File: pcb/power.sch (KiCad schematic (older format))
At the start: 46 parts, among them P11 CONN_01X01, P12 CONN_01X01, P8 CONN_01X06, P9 CONN_01X02, T1 NET-TIE, T2 NET-TIE, U1 TPS2420, U2 LT3487, U3 TPS63002, U7 TPS56x200, U8 LMZ10500

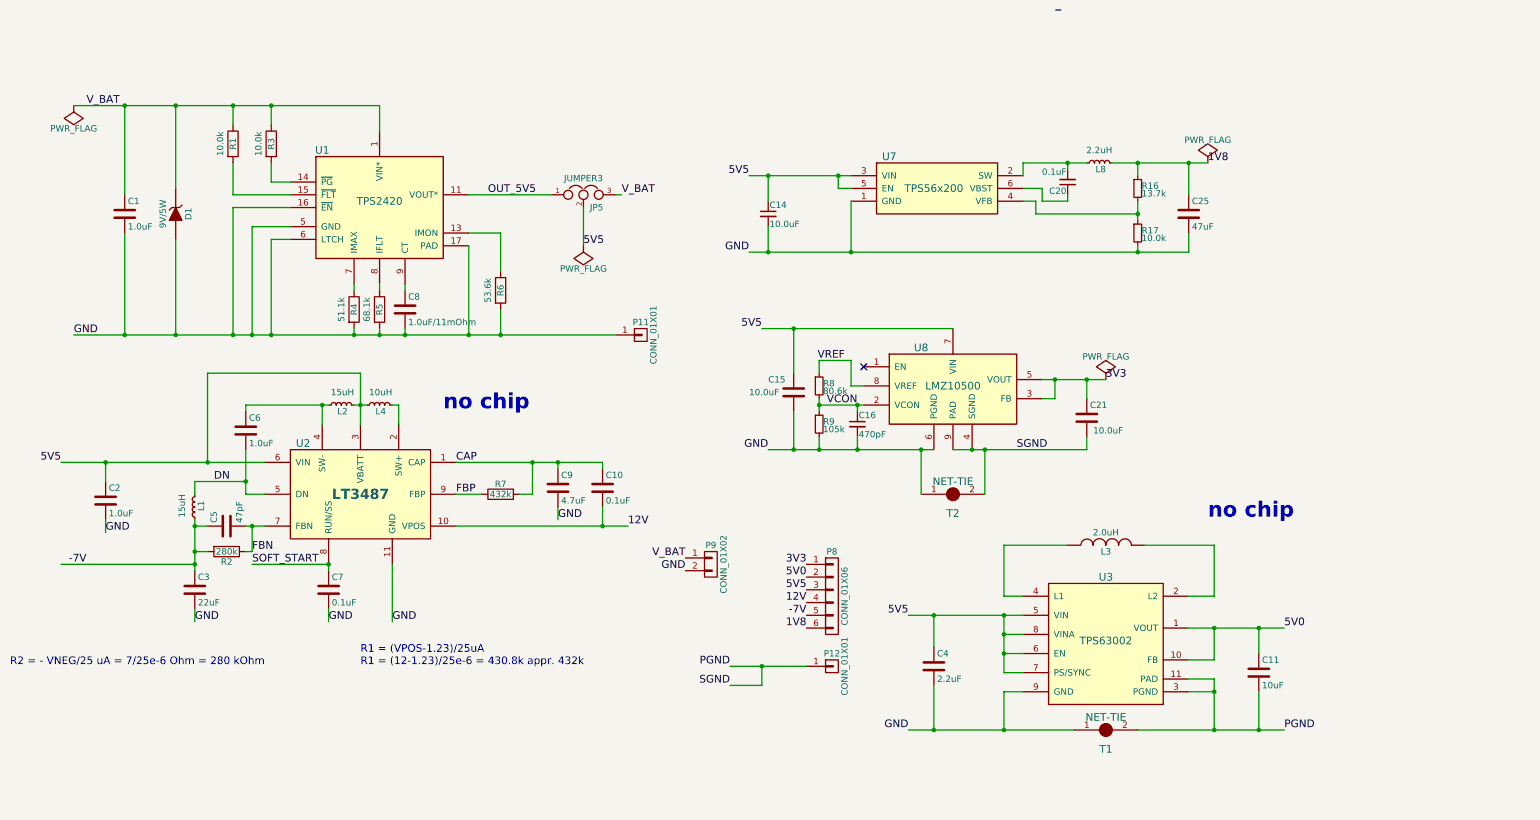
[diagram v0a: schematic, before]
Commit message: work
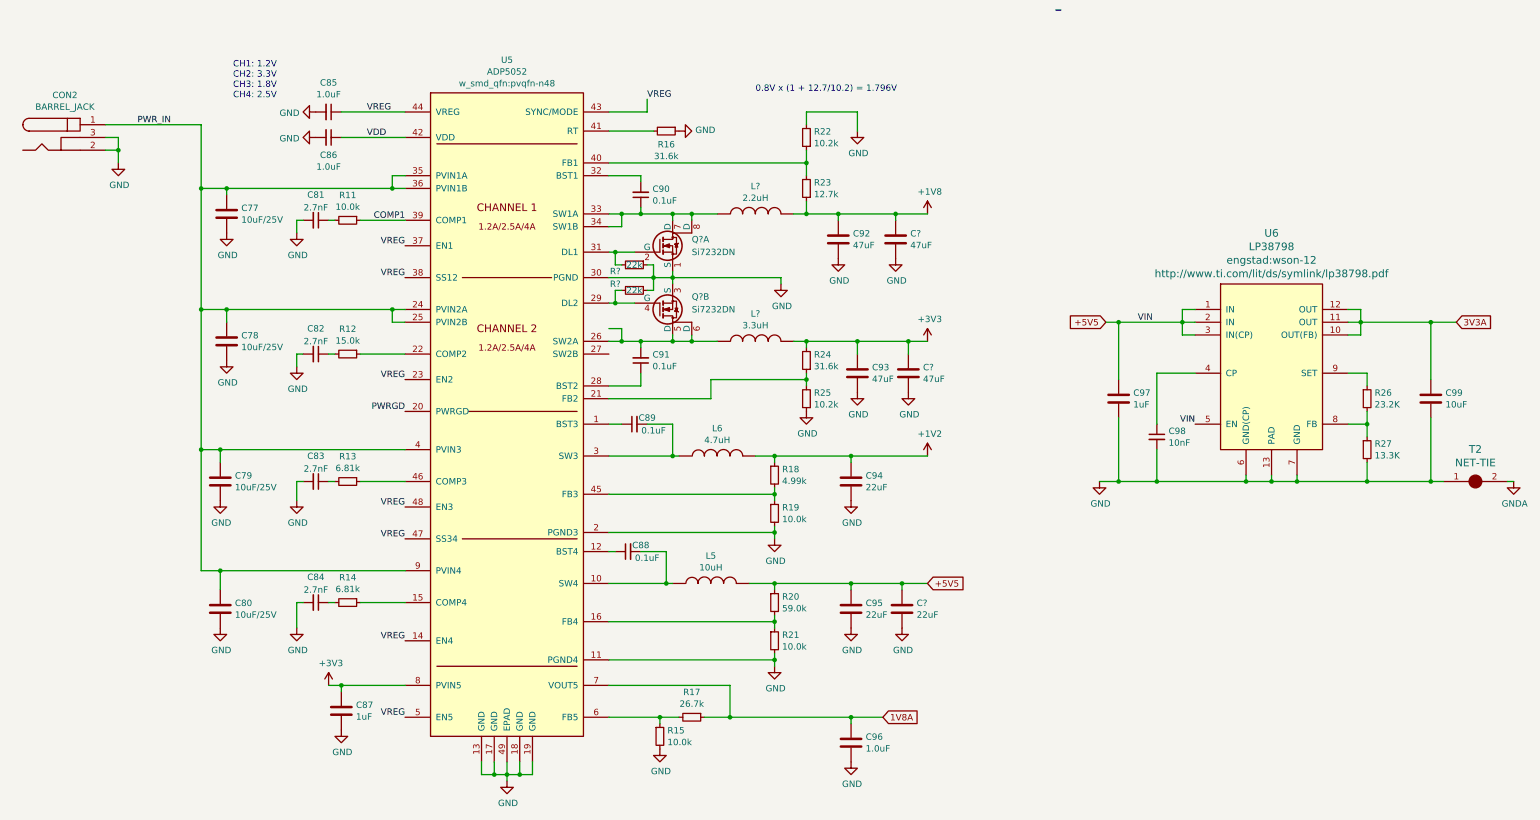
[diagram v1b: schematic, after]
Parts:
- removed C1, C2, C6: 1.0uF, Capacitors_SMD:C_0805_HandSoldering, symbol C
- removed C10, C7: 0.1uF, Capacitors_SMD:C_0805_HandSoldering, symbol C
- removed C11: 10uF, Capacitors_SMD:C_0805_HandSoldering, symbol C
- removed C14: 10.0uF, Capacitors_SMD:C_0805_HandSoldering, symbol C_Small
- removed C15, C21: 10.0uF, Capacitors_SMD:C_0805_HandSoldering, symbol C
- removed C16: 470pF, Capacitors_SMD:C_0402, symbol C_Small
- removed C20: 0.1uF, Capacitors_SMD:C_0603_HandSoldering, symbol C_Small
- removed C25: 47uF, Capacitors_SMD:C_1206_HandSoldering, symbol C
- removed C3: 22uF, Capacitors_SMD:C_0805_HandSoldering, symbol C
- removed C4: 2.2uF, Capacitors_SMD:C_0603_HandSoldering, symbol C
- removed C5: 47pF, Capacitors_SMD:C_0805_HandSoldering, symbol C
- removed C8: 1.0uF/11mOhm, Capacitors_SMD:C_0805_HandSoldering, symbol C
- removed C9: 4.7uF, Capacitors_SMD:C_0603_HandSoldering, symbol C
- removed D1: 9V/5W, Diodes_SMD:SMB_Standard, symbol ZENER
- removed JP5: JUMPER3, xess:xess-JP2, symbol JUMPER3
- removed L1, L2: 15uH, w_smd_inductors:inductor_smd_0805, symbol L_Small
- removed L3: 2.0uH, w_smd_inductors:inductor_smd_0805, symbol INDUCTOR
- removed L4: 10uH, w_smd_inductors:inductor_smd_0805, symbol L_Small
- removed L8: 2.2uH, w_smd_inductors:inductor_smd_0805, symbol L_Small
- removed P11, P12: CONN_01X01, xess:HDR_1x1, symbol CONN_01X01
- removed P8: CONN_01X06, Pin_Headers:Pin_Header_Straight_1x06, symbol CONN_01X06
- removed P9: CONN_01X02, Pin_Headers:Pin_Header_Straight_1x02, symbol CONN_01X02
- removed R1, R3: 10.0k, Resistors_SMD:R_0603_HandSoldering, symbol R
- removed R2: 280k, Resistors_SMD:R_0603_HandSoldering, symbol R
- removed R4: 51.1k, Resistors_SMD:R_0603_HandSoldering, symbol R
- removed R5: 68.1k, Resistors_SMD:R_0603_HandSoldering, symbol R
- removed R6: 53.6k, Resistors_SMD:R_0603_HandSoldering, symbol R
- removed R7: 432k, Resistors_SMD:R_0603_HandSoldering, symbol R
- removed R8: 80.6k, Resistors_SMD:R_0402, symbol R_Small
- removed R9: 105k, Resistors_SMD:R_0402, symbol R_Small
- removed T1: NET-TIE, Oddities:NetTie-I_SMD, symbol NET-TIE
- removed U1: TPS2420, Housings_DFN_QFN:QFN-16-1EP_4x4mm_Pitch0.65mm, symbol TPS2420
- removed U2: LT3487, w_smd_qfn:dfn10-3x3, symbol LT3487
- removed U3: TPS63002, Housings_DFN_QFN:DFN-10-1EP_3x3mm_Pitch0.5mm, symbol TPS63002
- removed U7: TPS56x200, Housings_SOT-23_SOT-143_TSOT-6:SOT-23-6, symbol TPS56x200
- removed U8: LMZ10500, engstad:llp-8, symbol LMZ10500
- added C77, C78, C79, C80: 10uF/25V, symbol C
- added C81, C82, C83, C84: 2.7nF, symbol C_Small
- added C85, C86: 1.0uF, symbol C_Small
- added C87: 1uF, symbol C
- added C88, C89, C90, C91: 0.1uF, symbol C_Small
- added C92, C93, C? (x2): 47uF, symbol C
- added C94, C95, C?: 22uF, symbol C
- added C96: 1.0uF, symbol C
- added C97: 1uF, engstad:0805, symbol C
- added C98: 10nF, engstad:0603, symbol C_Small
- added C99: 10uF, engstad:0805, symbol C
- added CON2: BARREL_JACK, symbol BARREL_JACK
- added L5: 10uH, symbol INDUCTOR
- added L6: 4.7uH, symbol INDUCTOR
- added L?: 3.3uH, symbol INDUCTOR
- added L?: 2.2uH, symbol INDUCTOR
- added Q? (x2): Si7232DN, POWERPAK-1212-8-DUAL, symbol Si7232DN
- added R11, R15, R19, R21: 10.0k, symbol R_Small
- added R12: 15.0k, symbol R_Small
- added R13, R14: 6.81k, symbol R_Small
- added R18: 4.99k, symbol R_Small
- added R20: 59.0k, symbol R_Small
- added R22, R25: 10.2k, symbol R_Small
- added R23: 12.7k, symbol R_Small
- added R24: 31.6k, symbol R_Small
- added R26: 23.2K, engstad:0603, symbol R_Small
- added R27: 13.3K, engstad:0603, symbol R_Small
- added R? (x2): 22k, symbol R_Small
- added U5: ADP5052, w_smd_qfn:pvqfn-n48, symbol ADP5052
- added U6: LP38798, engstad:wson-12, symbol LP38798
- R16: value 13.7k -> 31.6k; footprint Resistors_SMD:R_0402 -> (none)
- R17: value 10.0k -> 26.7k; footprint Resistors_SMD:R_0402 -> (none)
- T2: footprint Oddities:NetTie-I_Connected_SMD -> engstad:net-tie-0.5mm
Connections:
- net 1V8 is gone; now on net GND: R16.1
- net GND: now also C77.2, C78.2, C79.2, C80.2, C81.2, C82.2, C83.2, C84.2, C85.2, C86.2, C87.2, C92.2, C93.2, C94.2, C95.2, C96.2, C97.2, C98.2, C99.2, C?.2, C?.2, C?.2, CON2.2, CON2.3, Q?.1 (S), Q?.3 (S), R15.2, R19.2, R21.2, R22.2, R25.1, R27.2, R?.1, R?.1, U5.11 (PGND4), U5.13 (GND), U5.17 (GND), U5.18 (GND), U5.19 (GND), U5.2 (PGND3), U5.30 (PGND), U5.49 (EPAD), U6.13 (PAD), U6.6 (GND(CP)), U6.7 (GND); no longer R17.2
- net at R16.2: now also U5.41 (RT); no longer R17.1
- net PGND renamed GNDA
- new net: C89.1, U5.1 (BST3)
- new net: C88.2, L5.1, U5.10 (SW4)
- new net: C88.1, U5.12 (BST4)
- new net: R14.1, U5.15 (COMP4)
- new net: R20.2, R21.1, U5.16 (FB4)
- new net: R24.1, R25.2, U5.21 (FB2)
- new net: R12.1, U5.22 (COMP2)
- new net: C91.2, L?.1, Q?.5 (D), Q?.6 (D), U5.26 (SW2A)
- new net: C91.1, U5.28 (BST2)
- new net: Q?.4 (G), R?.2, U5.29 (DL2)
- new net: C89.2, L6.1, U5.3 (SW3)
- new net: Q?.2 (G), R?.2, U5.31 (DL1)
- new net: C90.2, U5.32 (BST1)
- new net: C90.1, L?.1, Q?.7 (D), Q?.8 (D), U5.33 (SW1A), U5.34 (SW1B)
- new net: R22.1, R23.2, U5.40 (FB1)
- new net: R18.2, R19.1, U5.45 (FB3)
- new net: R13.1, U5.46 (COMP3)
- new net: R15.1, R17.2, U5.6 (FB5)
- new net: C81.1, R11.2
- new net: C82.1, R12.2
- new net: C83.1, R13.2
- new net: C84.1, R14.2
- new net: C98.1, U6.4 (CP)
- new net: R26.2, R27.1, U6.8 (FB)
- new net: R26.1, U6.9 (SET)
- new net +1V2: C94.1, L6.2, R18.1
- new net +1V8: C92.1, C?.1, L?.2, R23.1
- new net +3V3: C87.1, C93.1, C?.1, L?.2, R24.2, U5.8 (PVIN5)
- new net +5V5: C95.1, C97.1, C?.1, L5.2, R20.1, U6.1 (IN), U6.2 (IN), U6.3 (IN(CP)), U6.5 (EN)
- new net 1V8A: C96.1, R17.1, U5.7 (VOUT5)
- new net 3V3A: C99.1, U6.10 (OUT(FB)), U6.11 (OUT), U6.12 (OUT)
- new net COMP1: R11.1, U5.39 (COMP1)
- new net PWRGD: U5.20 (PWRGD)
- new net PWR_IN: C77.1, C78.1, C79.1, C80.1, CON2.1, U5.24 (PVIN2A), U5.25 (PVIN2B), U5.35 (PVIN1A), U5.36 (PVIN1B), U5.4 (PVIN3), U5.9 (PVIN4)
- new net VDD: C86.1, U5.42 (VDD)
- new net VREG: C85.1, U5.14 (EN4), U5.23 (EN2), U5.37 (EN1), U5.38 (SS12), U5.43 (SYNC/MODE), U5.44 (VREG), U5.47 (SS34), U5.48 (EN3), U5.5 (EN5)
- no-connect marks 1 -> 0
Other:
- note added: "0.8V x (1 + 12.7/10.2) = 1.796V"
- note added: "CH1: 1.2V\nCH2: 3.3V\nCH3: 1.8V\nCH4: 2.5V"
- note removed: "R1 = (VPOS-1.23)/25uA \nR1 = (12-1.23)/25e-6 = 430.8k appr. 432k"
- note removed: "R2 = - VNEG/25 uA = 7/25e-6 Ohm = 280 kOhm"
- note removed: "no chip\n"
